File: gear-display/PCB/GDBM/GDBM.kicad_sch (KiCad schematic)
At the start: 3 parts, among them J1 Con_Screw_1x04_691313510004, J2 Con_Screw_1x04_691313510004

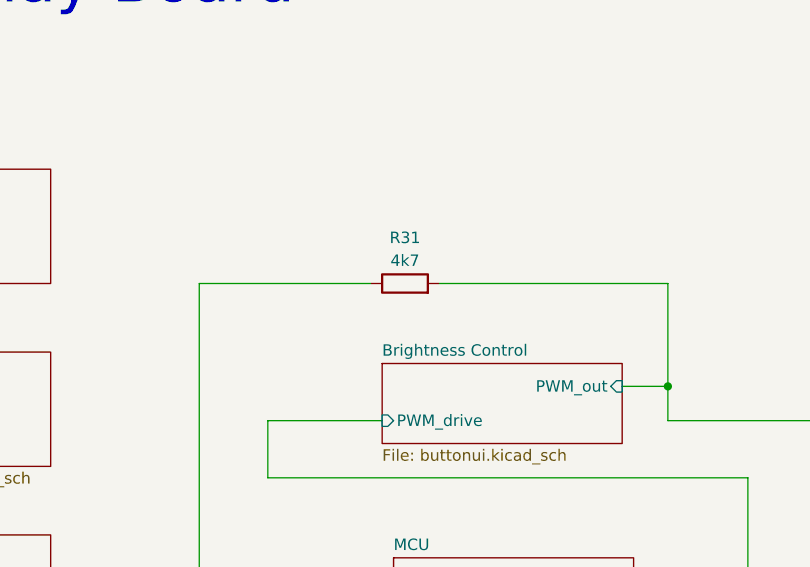
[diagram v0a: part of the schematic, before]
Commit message: Layout
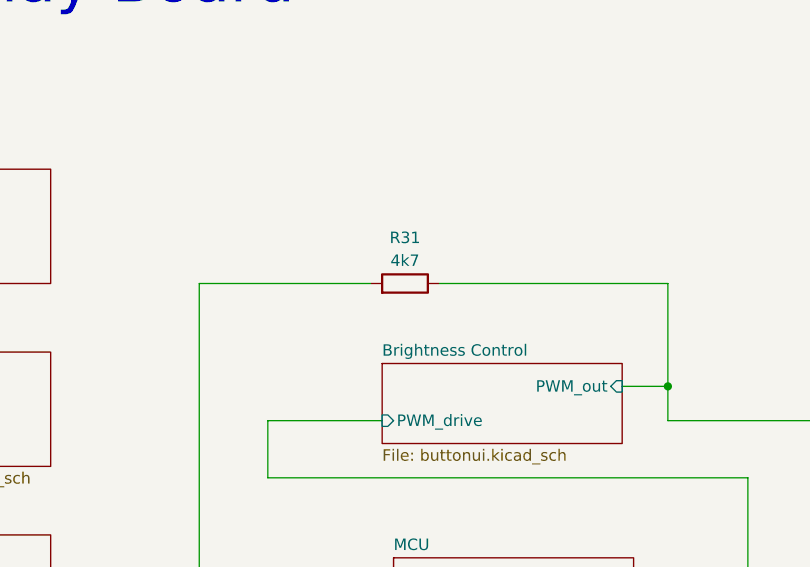
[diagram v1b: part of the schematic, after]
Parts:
- J1, J2: value Con_Screw_1x04_691313510004 -> 1x04
- R31: value R_0402_4700_1% -> 4k7
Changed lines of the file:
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@@
       (effects (font (size 1.27 1.27)))
     )
-    (property "Value" "Con_Screw_1x04_691313510004" (at 250.19 195.58 0)
+    (property "Value" "1x04" (at 250.19 195.58 0)
       (effects (font (size 1.27 1.27)) (justify left) hide)
     )
@@
       (effects (font (size 1.27 1.27)))
     )
-    (property "Value" "R_0402_4700_1%" (at 72.39 68.58 0)
+    (property "Value" "4k7" (at 72.39 68.58 0)
       (effects (font (size 1.27 1.27)) (justify left) hide)
     )
@@
       (effects (font (size 1.27 1.27)))
     )
-    (property "Value" "Con_Screw_1x04_691313510004" (at 60.96 196.85 0)
+    (property "Value" "1x04" (at 60.96 196.85 0)
       (effects (font (size 1.27 1.27)) (justify left) hide)
     )
